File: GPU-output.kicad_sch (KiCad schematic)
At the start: 23 parts, among them J1 Conn_1-2212115-4, Q1 BSS138PW, Q2 SI7613DN-T1-GE3, Q3 SI7613DN-T1-GE3, U4 TMCS1100A2-Q1

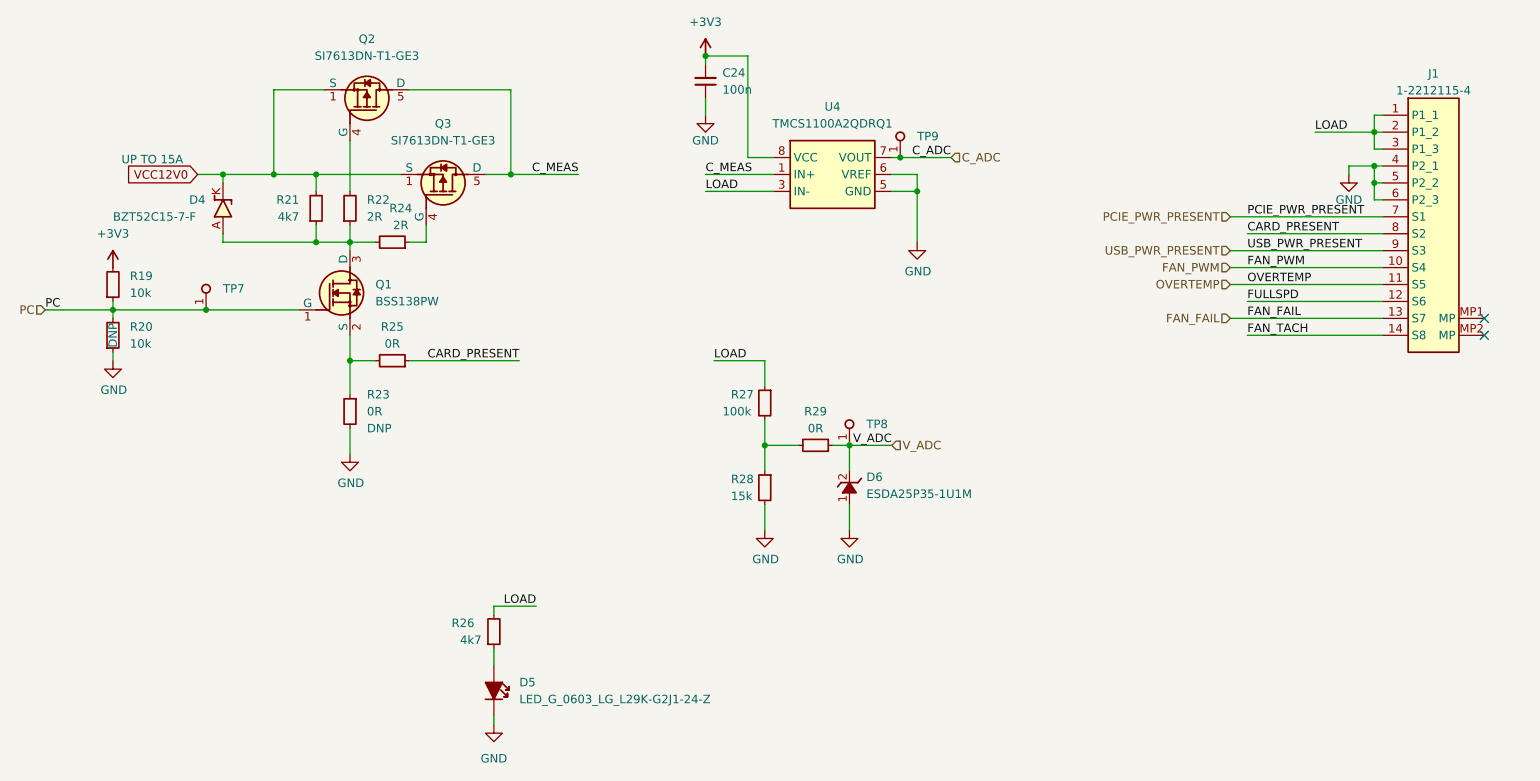
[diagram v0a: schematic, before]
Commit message: Start routing of GPIO/ADC circuit
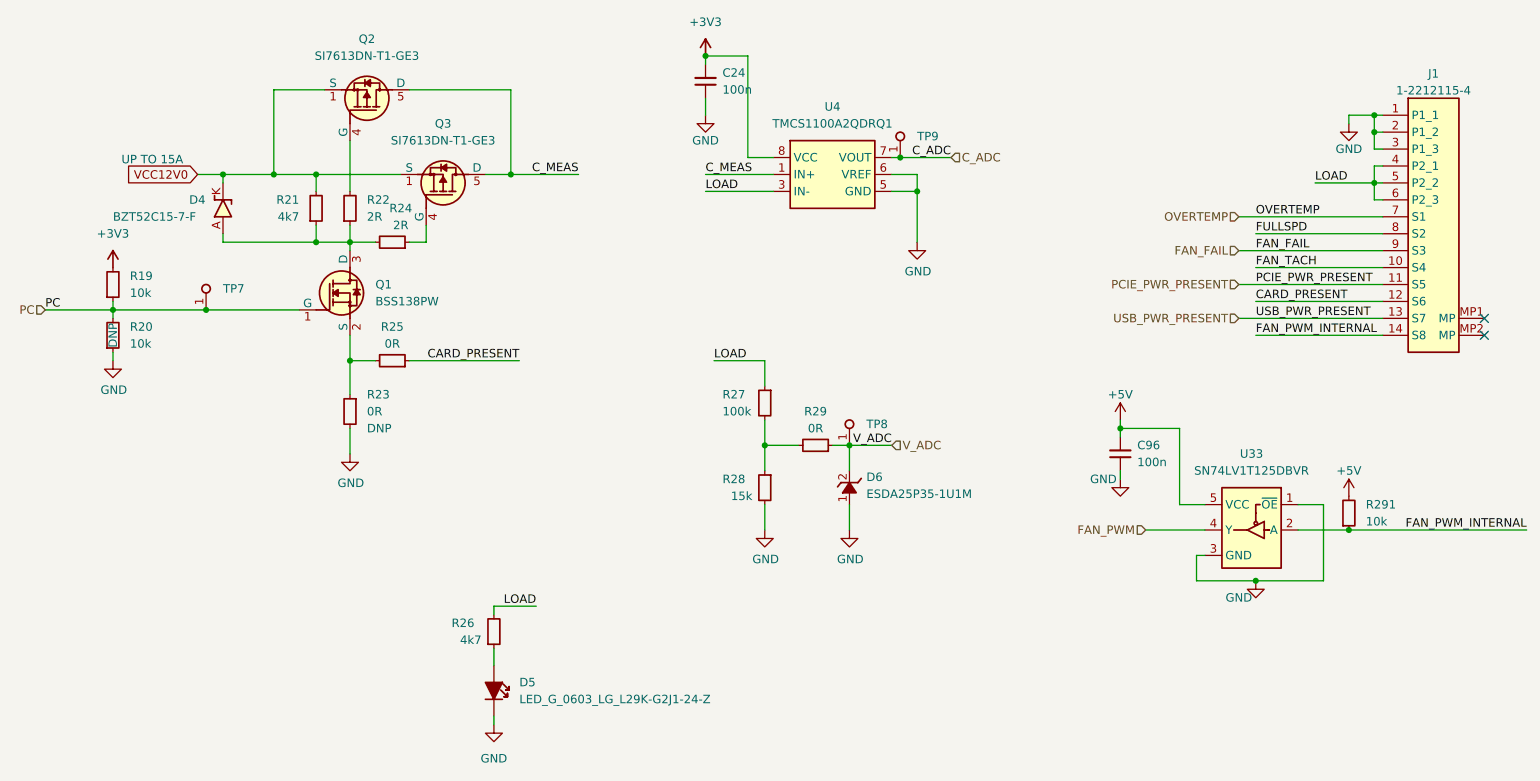
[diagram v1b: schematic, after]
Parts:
- added C96: C_100n_0402, antmicro-footprints:C_0402_1005Metric, symbol antmicroCapacitors0402:C_100n_0402
- added R291: R_10k_0402, antmicro-footprints:R_0402_1005Metric, symbol antmicroResistors0402:R_10k_0402
- added U33: SN74LV1T125DBVR, antmicro-footprints:SOT-23-5, symbol antmicroLogicBuffersDriversReceiversTransceivers:SN74LV1T125DBVR
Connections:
- net CARD_PRESENT: now also J1.12 (S6); no longer J1.8 (S2)
- net FAN_FAIL: now also J1.9 (S3); no longer J1.13 (S7)
- net FAN_PWM: now also U33.4 (Y); no longer J1.10 (S4)
- net FAN_TACH: now also J1.10 (S4); no longer J1.14 (S8)
- net FULLSPD: now also J1.8 (S2); no longer J1.12 (S6)
- net GND: now also J1.1 (P1_1), J1.2 (P1_2), J1.3 (P1_3), C96.1, U33.1 (~{OE}), U33.3 (GND); no longer J1.4 (P2_1), J1.5 (P2_2), J1.6 (P2_3)
- net LOAD: now also J1.4 (P2_1), J1.5 (P2_2), J1.6 (P2_3); no longer J1.1 (P1_1), J1.2 (P1_2), J1.3 (P1_3)
- net OVERTEMP: now also J1.7 (S1); no longer J1.11 (S5)
- net PCIE_PWR_PRESENT: now also J1.11 (S5); no longer J1.7 (S1)
- net USB_PWR_PRESENT: now also J1.13 (S7); no longer J1.9 (S3)
- new net +5V: C96.2, R291.2, U33.5 (VCC)
- new net FAN_PWM_INTERNAL: J1.14 (S8), R291.1, U33.2 (A)
